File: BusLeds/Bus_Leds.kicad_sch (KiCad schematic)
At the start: 19 parts, among them J1 Conn_01x02, J4 Conn_01x02, J48 Conn_01x08

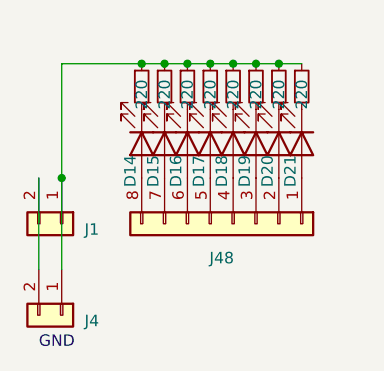
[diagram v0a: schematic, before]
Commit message: Updated Footprint
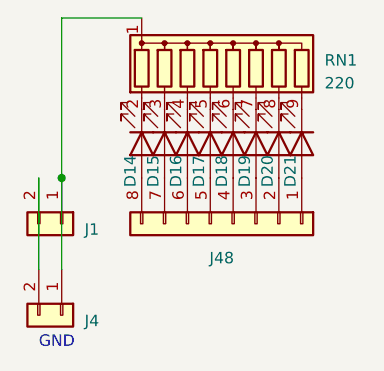
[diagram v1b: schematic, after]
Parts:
- removed R10, R11, R12, R13, R6, R7, R8, R9: 220, symbol Device:R_Small
- added RN1: 220, Resistor_THT:R_Array_SIP9, symbol Device:R_Network08
- D14, D15, D16, D17, D18, D19, D20, D21: footprint (none) -> LED_THT:LED_D5.0mm-3
- J1, J4: footprint (none) -> Connector_PinHeader_2.54mm:PinHeader_1x02_P2.54mm_Vertical
- J48: footprint (none) -> Connector_PinHeader_2.54mm:PinHeader_1x08_P2.54mm_Vertical
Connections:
- net at J1.1 (Pin_1), J4.1 (Pin_1): now also RN1.1 (common)
- net at D15.1 (K): now also RN1.3 (R2)
- net at D16.1 (K): now also RN1.4 (R3)
- net at D14.1 (K): now also RN1.2 (R1)
- net at D19.1 (K): now also RN1.7 (R6)
- net at D20.1 (K): now also RN1.8 (R7)
- net at D18.1 (K): now also RN1.6 (R5)
- net at D21.1 (K): now also RN1.9 (R8)
- net at D17.1 (K): now also RN1.5 (R4)
